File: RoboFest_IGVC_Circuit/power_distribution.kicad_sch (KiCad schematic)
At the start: 9 parts, among them J1 E-stop, J2 E-stop relay, J3 Wireless E-stop RF relay, J4 Buck converter #1 (5V/5A, Pi 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, J5 Buck converter #2 (5V/3A, sen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, J6 Buck converter #3 (5-6V, serv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, U3 INA219AxD

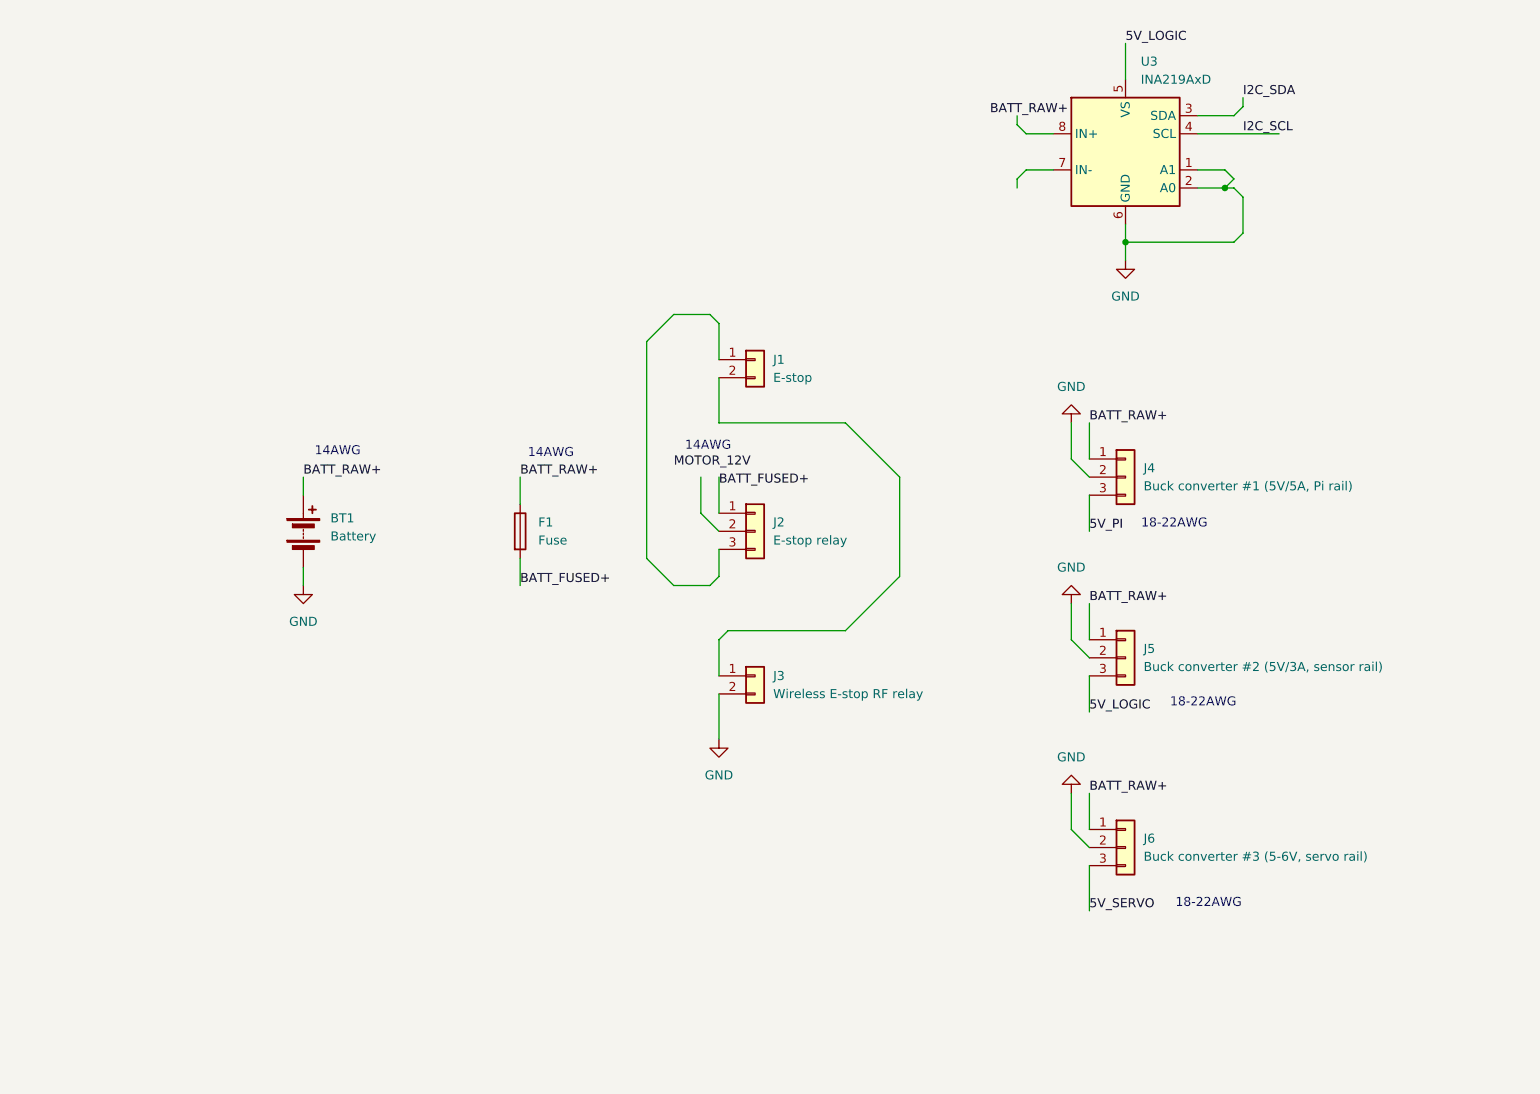
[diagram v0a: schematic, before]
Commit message: updated diagram
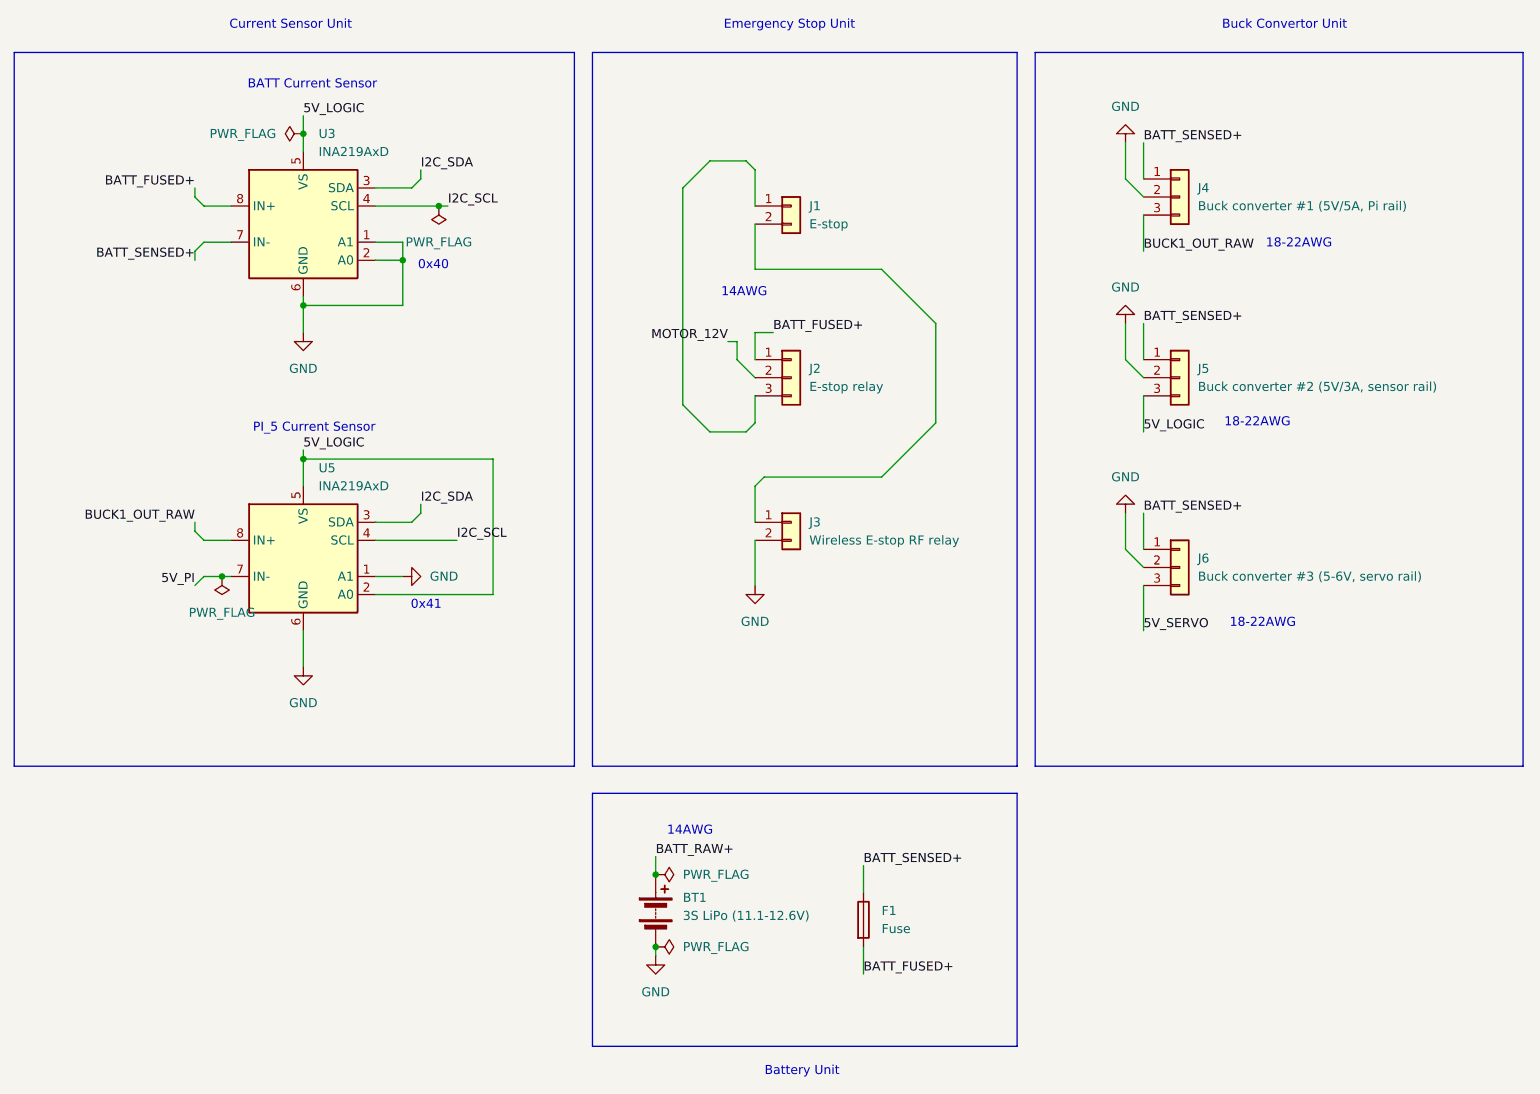
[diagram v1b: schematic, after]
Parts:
- added U5: INA219AxD, Package_SO:SOIC-8_3.9x4.9mm_P1.27mm, symbol Sensor_Energy:INA219AxD
- BT1: value Battery -> 3S LiPo (11.1-12.6V)
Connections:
- net 5V_LOGIC: now also U5.2 (A0), U5.5 (VS)
- net 5V_PI: now also U5.7 (IN-); no longer J4.3 (Pin_3)
- net BATT_FUSED+: now also U3.8 (IN+)
- net BATT_RAW+: no longer F1.1, J4.1 (Pin_1), J5.1 (Pin_1), J6.1 (Pin_1)
- net GND: now also U5.1 (A1), U5.6 (GND)
- net I2C_SCL: now also U5.4 (SCL)
- net I2C_SDA: now also U5.3 (SDA)
- net MOTOR_12V: now also J2.2 (Pin_2)
- net BATT_SENSED+: now reaches U3.7 (IN-)
- net BATT_SENSED+: now also F1.1, J4.1 (Pin_1), J5.1 (Pin_1), J6.1 (Pin_1)
- new net BUCK1_OUT_RAW: J4.3 (Pin_3), U5.8 (IN+)
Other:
- note added: "0x40"
- note added: "0x41"
- note added: "BATT Current Sensor"
- note added: "Battery Unit"
- note added: "Buck Convertor Unit"
- note added: "Current Sensor Unit"
- note added: "Emergency Stop Unit"
- note added: "PI_5 Current Sensor"
- moved on the sheet: BT1, F1, J1, J2, J3, J4, J5, J6, U3
